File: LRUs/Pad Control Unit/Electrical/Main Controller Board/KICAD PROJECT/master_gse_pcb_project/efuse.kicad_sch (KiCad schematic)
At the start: 19 parts, among them J4 B2B-XH-A, U3 TPS259830ONRGER

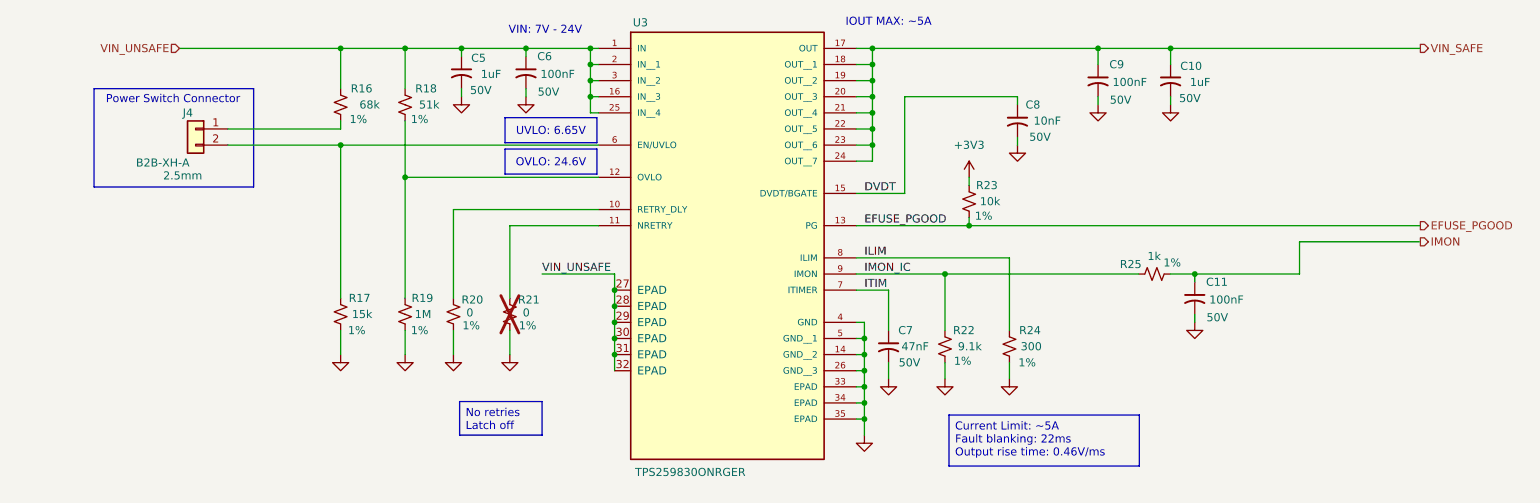
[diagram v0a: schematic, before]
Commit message: Committttt
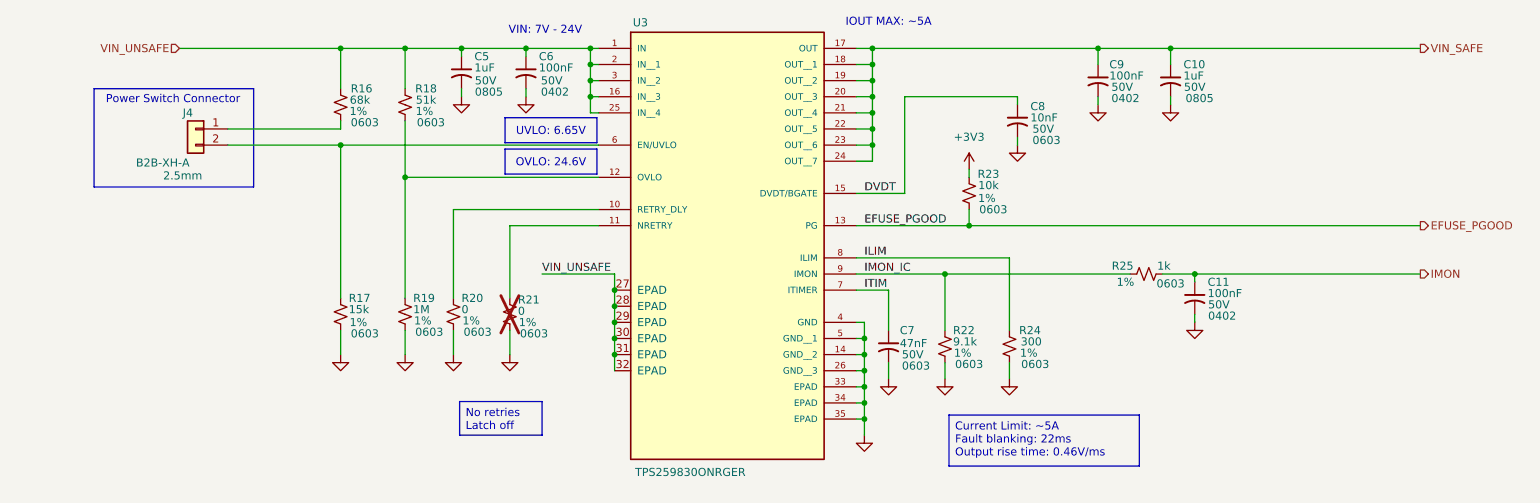
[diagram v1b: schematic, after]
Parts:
- C10, C5: Footprint_Size (none) -> 0805
- C11, C6, C9: Footprint_Size (none) -> 0402
- C7, C8, R16, R17, R18, R19, R20, R21, R22, R23, R24, R25: Footprint_Size (none) -> 0603
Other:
- moved on the sheet: R23, R25

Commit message: Commit da changes
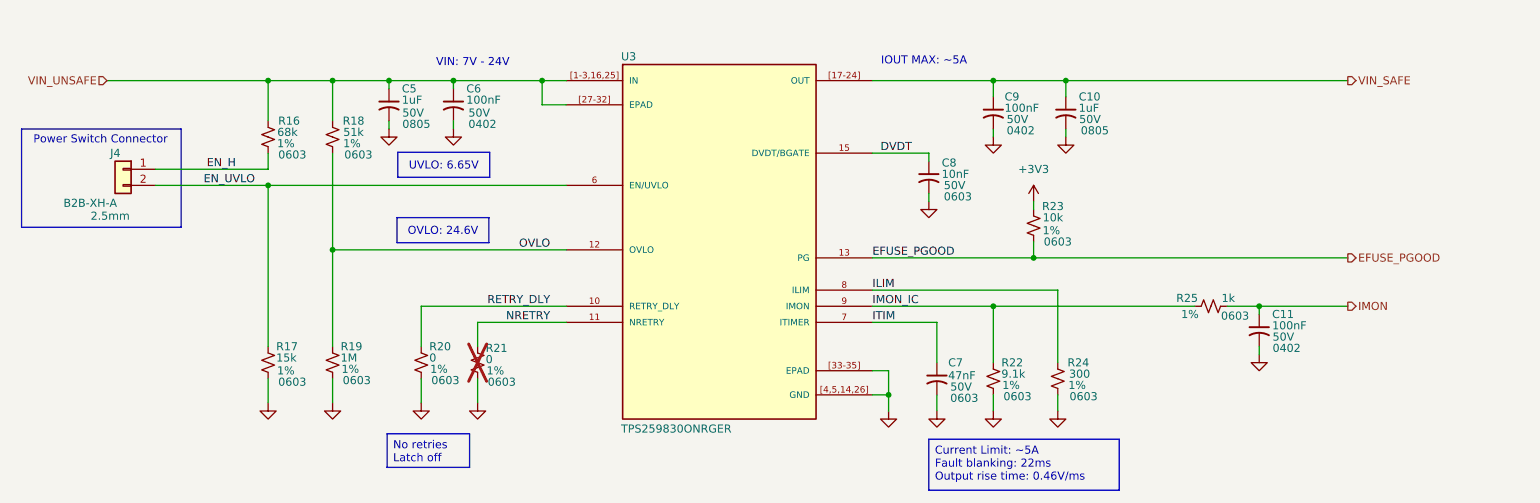
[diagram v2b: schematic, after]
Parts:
- U3: JLCPCB Part # C20611808 -> (none)
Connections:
- net GND: now also U3.[33-35] (EPAD), U3.[4,5,14,26] (GND); no longer U3.14 (GND__2), U3.26 (GND__3), U3.33 (EPAD), U3.34 (EPAD), U3.35 (EPAD), U3.4 (GND), U3.5 (GND__1)
- net VIN_SAFE: now also U3.[17-24] (OUT); no longer U3.17 (OUT), U3.18 (OUT__1), U3.19 (OUT__2), U3.20 (OUT__3), U3.21 (OUT__4), U3.22 (OUT__5), U3.23 (OUT__6), U3.24 (OUT__7)
- net VIN_UNSAFE: now also U3.[1-3,16,25] (IN), U3.[27-32] (EPAD); no longer U3.1 (IN), U3.16 (IN__3), U3.2 (IN__1), U3.25 (IN__4), U3.27 (EPAD), U3.28 (EPAD), U3.29 (EPAD), U3.3 (IN__2), U3.30 (EPAD), U3.31 (EPAD), U3.32 (EPAD)
- net OVLO: now reaches R18.2, R19.2, U3.12 (OVLO)
- net EN_H: now reaches J4.1 (Pin_1), R16.2
- net EN_UVLO: now reaches J4.2 (Pin_2), R17.2, U3.6 (EN/UVLO)
- net RETRY_DLY: now reaches R20.2, U3.10 (RETRY_DLY)
- net NRETRY: now reaches R21.2, U3.11 (NRETRY)
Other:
- moved on the sheet: C10, C11, C5, C6, C7, C8, C9, J4, R16, R17, R18, R19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
